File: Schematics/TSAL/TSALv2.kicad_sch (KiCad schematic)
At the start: 21 parts, among them J1 043045-0412, Q1 BS250P, Q2 BS170, Q3 UJ3N120035K3S, Q4 BS170, U1 H11L1M

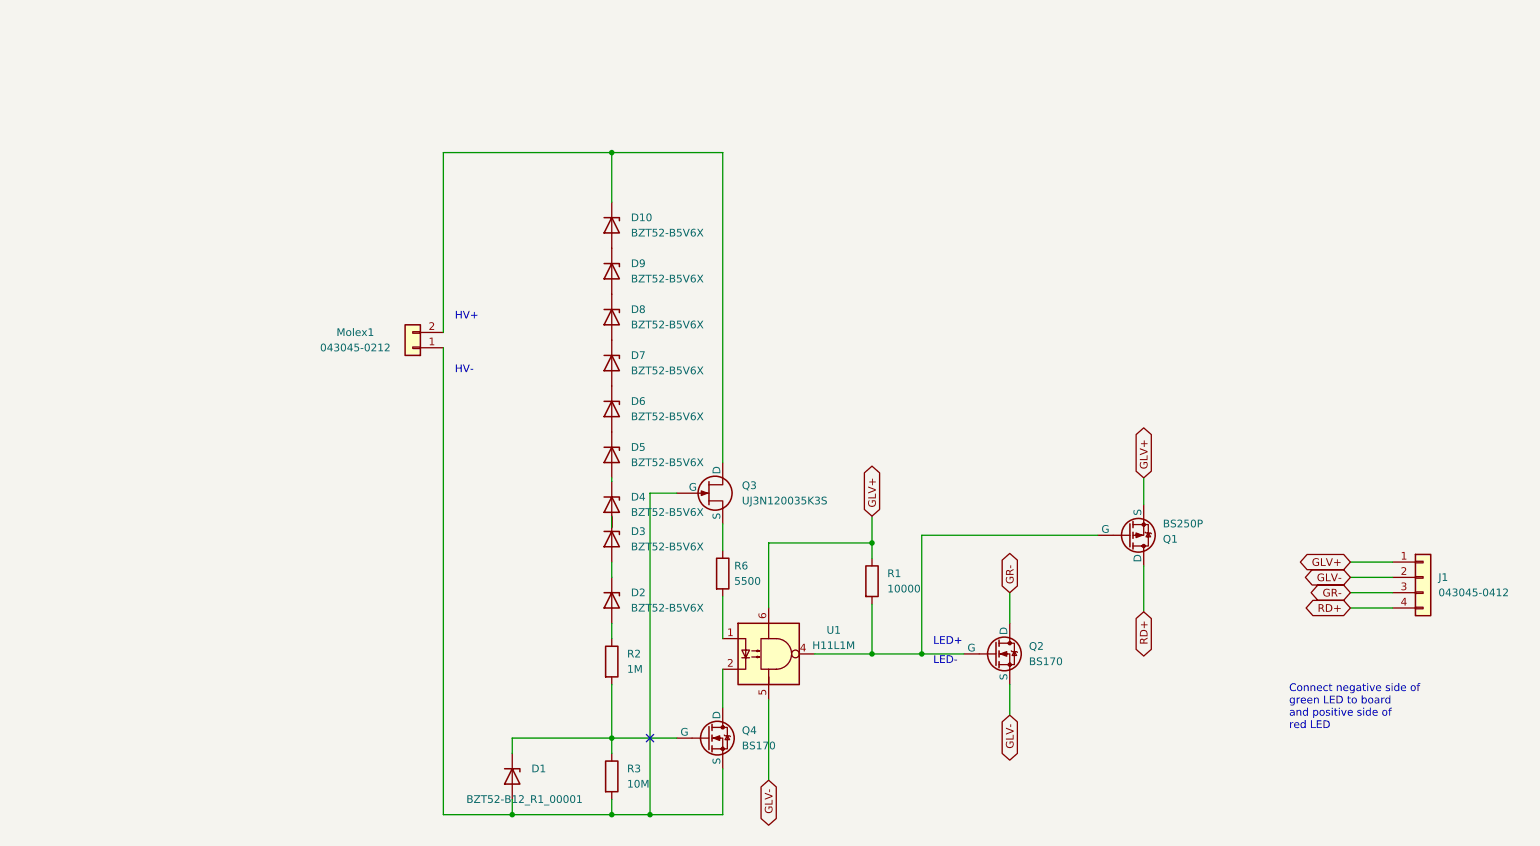
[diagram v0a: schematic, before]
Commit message: edits
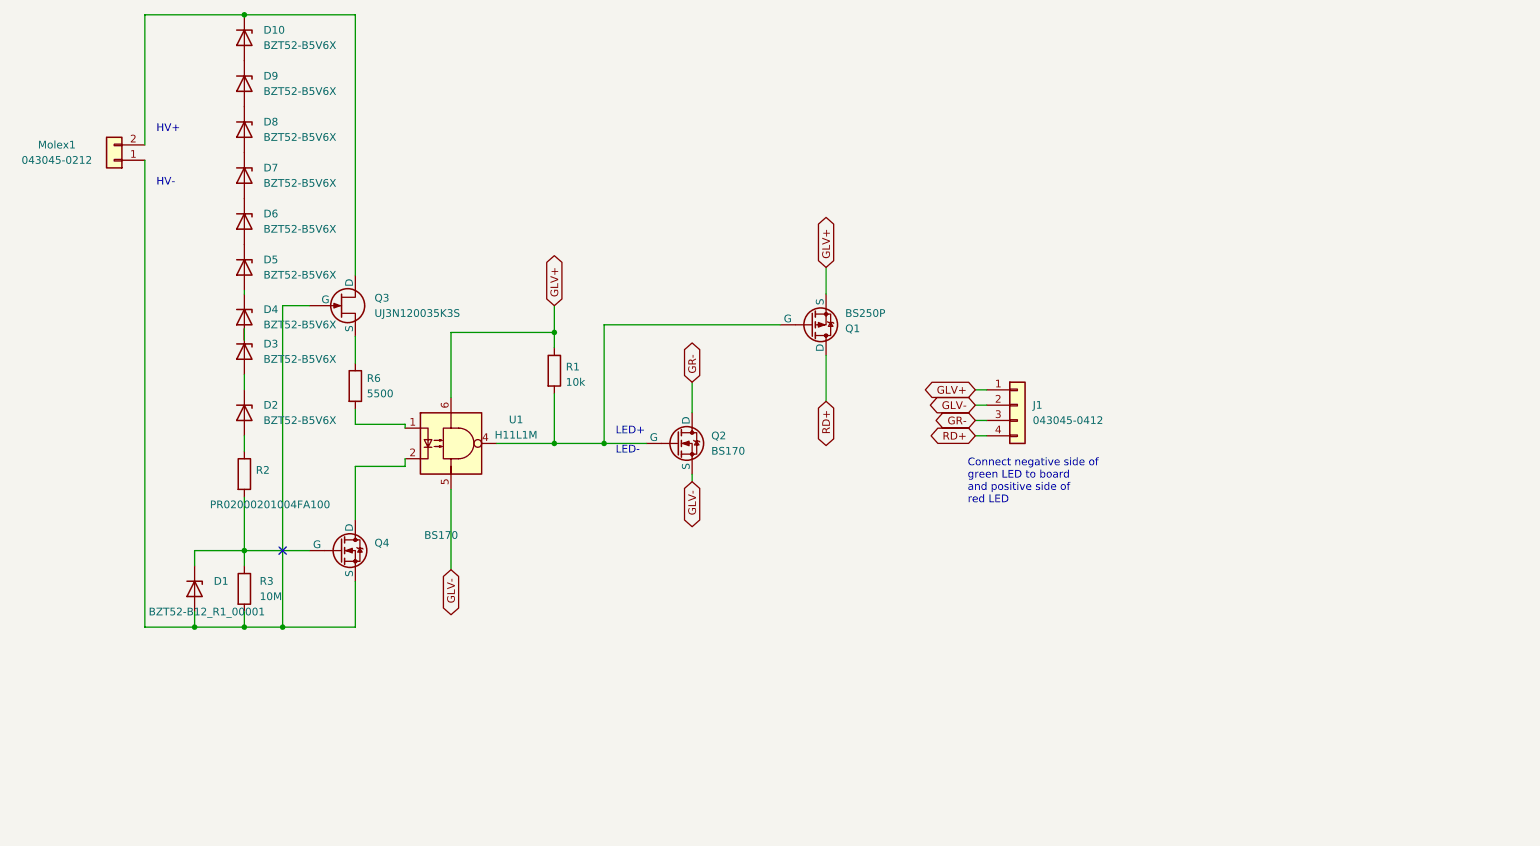
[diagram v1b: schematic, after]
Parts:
- R1: value 10000 -> 10k
- R2: value 1M -> PR02000201004FA100
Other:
- moved on the sheet: D1, D10, D2, D3, D4, D5, D6, D7, D8, D9, J1, Molex1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
